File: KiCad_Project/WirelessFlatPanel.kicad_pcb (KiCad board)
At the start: 2 copper layers, 61.2 x 51.3 mm, 16 parts, among them Q1 Val**

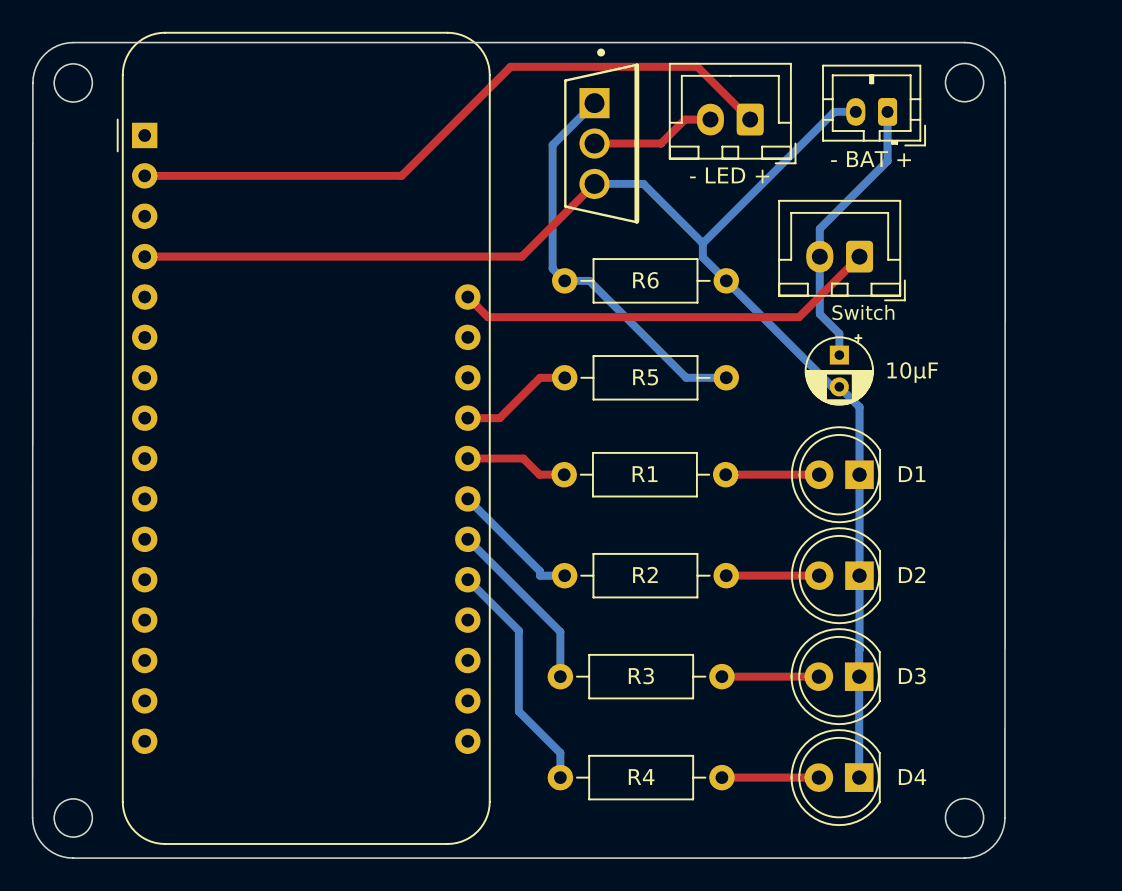
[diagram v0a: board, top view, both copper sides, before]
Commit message: Updated KiCad project
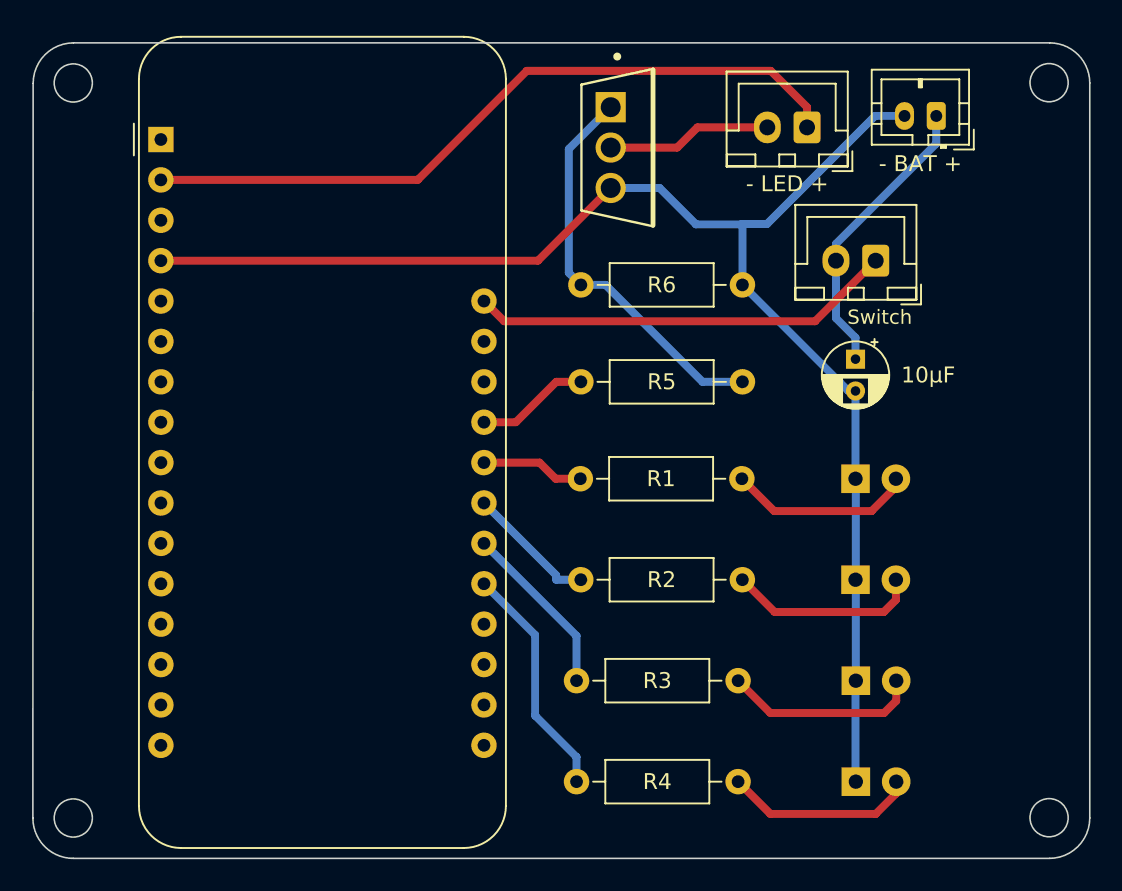
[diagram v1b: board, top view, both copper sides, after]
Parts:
- D1, D2, D3, D4: moved to B.Cu
- moved - LED + 3.61 mm to (150.6, 66.3)
- moved - BAT + 3.07 mm to (158.8, 65.6)
- moved A1 1.05 mm to (110.0, 67.1)
- moved R2 1.05 mm to (146.6, 94.7)
- moved R3 1.05 mm to (146.3, 101.1)
- moved R5 1.05 mm to (146.6, 82.3)
- moved R6 1.05 mm to (146.6, 76.2)
- moved Switch 1.05 mm to (154.9, 74.7)
- moved 10µF 1.05 mm to (153.7, 80.9)
- moved Q1 1.05 mm to (138.7, 67.6)
- moved R1 1.05 mm to (146.5, 88.4)
- moved R4 1.05 mm to (146.3, 107.4)
- moved D2 0.36 mm to (153.7, 94.7), turned to 0 degrees
- moved D1 0.36 mm to (153.7, 88.4), turned to 0 degrees
- moved D3 0.33 mm to (153.7, 101.1), turned to 0 degrees
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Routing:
- net Net-(D3-Pad2): track 6.10 -> 12.4 mm
- net Net-(D2-Pad2): track 5.85 -> 12.1 mm
- net Net-(D4-Pad2): track 6.10 -> 12.1 mm
- net Net-(D1-Pad2): track 5.88 -> 11.7 mm
- net Net-(A1-Pad2): track 42.3 -> 45.7 mm
- net Net-(Q1-Pad2): track 7.91 -> 10.4 mm
- net GND: track 89.5 -> 90.7 mm
- net Net-(C1-Pad1): track 17.6 -> 18.4 mm
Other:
- board size 61.2 x 51.3 mm -> 66.5 x 51.3 mm
